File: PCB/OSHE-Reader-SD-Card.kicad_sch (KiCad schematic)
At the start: 2 parts, among them J2 112L-TDA0

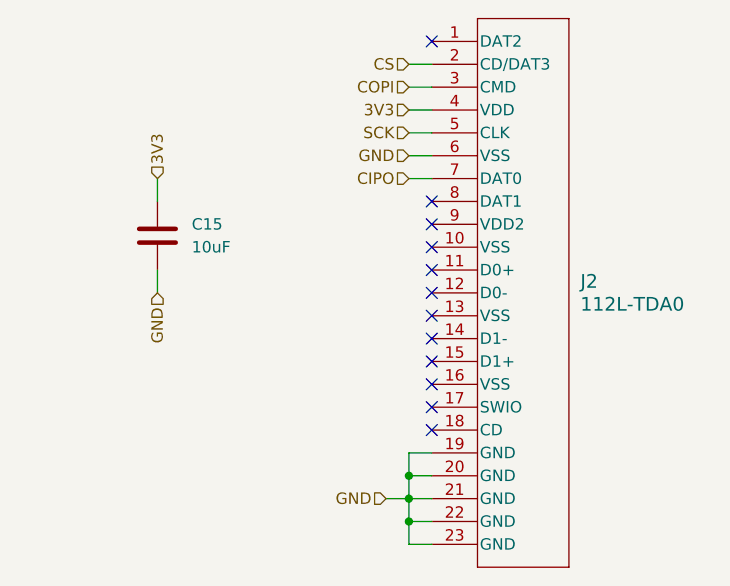
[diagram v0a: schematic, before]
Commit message: HOPEFULLY GOOD FOR EVER (good for first semester) :)
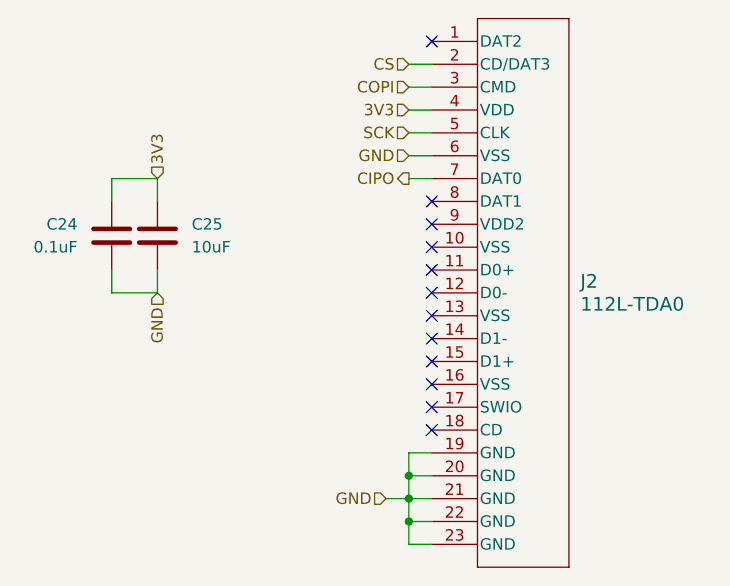
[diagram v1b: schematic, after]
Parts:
- added C24: 0.1uF, symbol Device:C
- J2: footprint CONN_112L-TDA0_ATT -> 112L_TDA0:CONN_112L-TDA0_ATT
- renumbered C15 to C25
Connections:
- net 3V3: now also C24.1
- net GND: now also C24.2
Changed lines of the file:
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@@
+	(wire
+		(pts
+			(xy 39.37 67.31) (xy 39.37 64.77)
+		)
+		(stroke
+			(width 0)
+			(type default)
+		)
+	)
 	(wire
 		(pts
@@
 	(wire
 		(pts
+			(xy 39.37 77.47) (xy 44.45 77.47)
+		)
+		(stroke
+			(width 0)
+			(type default)
+		)
+	)
+	(wire
+		(pts
 			(xy 69.85 100.33) (xy 72.39 100.33)
 		)
@@
 	(wire
 		(pts
+			(xy 39.37 64.77) (xy 44.45 64.77)
+		)
+		(stroke
+			(width 0)
+			(type default)
+		)
+	)
+	(wire
+		(pts
 			(xy 72.39 52.07) (xy 74.93 52.07)
 		)
@@
 	(wire
 		(pts
+			(xy 39.37 74.93) (xy 39.37 77.47)
+		)
+		(stroke
+			(width 0)
+			(type default)
+		)
+	)
+	(wire
+		(pts
 			(xy 72.39 59.69) (xy 74.93 59.69)
 		)
@@
 	)
 	(hierarchical_label "CIPO"
-		(shape input)
+		(shape output)
 		(at 72.39 64.77 180)
 		(effects
@@
 			)
 			(justify right)
+		)
+	)
+	(symbol
+		(lib_id "Device:C")
+		(at 39.37 71.12 0)
+		(mirror y)
+		(unit 1)
+		(exclude_from_sim no)
+		(in_bom yes)
+		(on_board yes)
+		(dnp no)
+		(property "Reference" "C24"
+			(at 35.56 69.8499 0)
+			(effects
+				(font
+					(size 1.27 1.27)
+				)
+				(justify left)
+			)
+		)
+		(property "Value" "0.1uF"
+			(at 35.56 72.3899 0)
+			(effects
+				(font
+					(size 1.27 1.27)
+				)
+				(justify left)
+			)
+		)
+		(property "Footprint" ""
+			(at 38.4048 74.93 0)
+			(effects
+				(font
+					(size 1.27 1.27)
+				)
+				(hide yes)
+			)
+		)
+		(property "Datasheet" "~"
+			(at 39.37 71.12 0)
+			(effects
+				(font
+					(size 1.27 1.27)
+				)
+				(hide yes)
+			)
+		)
+		(property "Description" "Unpolarized capacitor"
+			(at 39.37 71.12 0)
+			(effects
+				(font
+					(size 1.27 1.27)
+				)
+				(hide yes)
+			)
+		)
+		(pin "1"
+		)
+		(pin "2"
+		)
+		(instances
+			(project "OSHE-Reader-PCB"
+				(path "/3f072c92-e35a-4654-839b-728bd3dc3a46/f673c940-d558-4160-83eb-d33ca6356616"
+					(reference "C24")
+					(unit 1)
+				)
+			)
 		)
 	)
@@
 			)
 		)
-		(property "Footprint" "CONN_112L-TDA0_ATT"
+		(property "Footprint" "112L_TDA0:CONN_112L-TDA0_ATT"
 			(at 69.85 49.53 0)
 			(effects
@@
 		(dnp no)
 		(fields_autoplaced yes)
-		(property "Reference" "C15"
+		(property "Reference" "C25"
 			(at 48.26 69.8499 0)
 			(effects
@@
 			(project ""
 				(path "/3f072c92-e35a-4654-839b-728bd3dc3a46/f673c940-d558-4160-83eb-d33ca6356616"
-					(reference "C15")
+					(reference "C25")
 					(unit 1)
 				)

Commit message: small
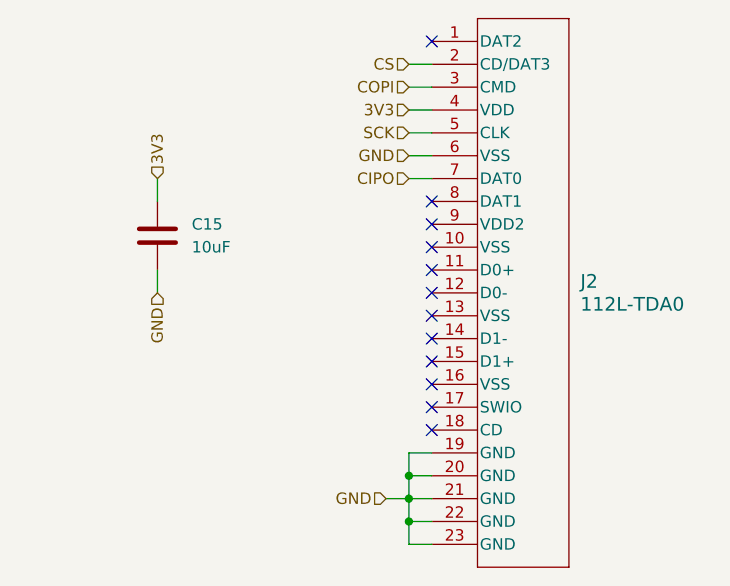
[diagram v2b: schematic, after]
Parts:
- removed C24: 0.1uF, symbol Device:C
- J2: footprint 112L_TDA0:CONN_112L-TDA0_ATT -> CONN_112L-TDA0_ATT
- renumbered C25 to C15
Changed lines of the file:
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@@
-	(wire
-		(pts
-			(xy 39.37 67.31) (xy 39.37 64.77)
-		)
-		(stroke
-			(width 0)
-			(type default)
-		)
-	)
 	(wire
 		(pts
@@
 	(wire
 		(pts
-			(xy 39.37 77.47) (xy 44.45 77.47)
-		)
-		(stroke
-			(width 0)
-			(type default)
-		)
-	)
-	(wire
-		(pts
 			(xy 69.85 100.33) (xy 72.39 100.33)
 		)
@@
 	(wire
 		(pts
-			(xy 39.37 64.77) (xy 44.45 64.77)
-		)
-		(stroke
-			(width 0)
-			(type default)
-		)
-	)
-	(wire
-		(pts
 			(xy 72.39 52.07) (xy 74.93 52.07)
 		)
@@
 	(wire
 		(pts
-			(xy 39.37 74.93) (xy 39.37 77.47)
-		)
-		(stroke
-			(width 0)
-			(type default)
-		)
-	)
-	(wire
-		(pts
 			(xy 72.39 59.69) (xy 74.93 59.69)
 		)
@@
 	)
 	(hierarchical_label "CIPO"
-		(shape output)
+		(shape input)
 		(at 72.39 64.77 180)
 		(effects
@@
 			)
 			(justify right)
-		)
-	)
-	(symbol
-		(lib_id "Device:C")
-		(at 39.37 71.12 0)
-		(mirror y)
-		(unit 1)
-		(exclude_from_sim no)
-		(in_bom yes)
-		(on_board yes)
-		(dnp no)
-		(property "Reference" "C24"
-			(at 35.56 69.8499 0)
-			(effects
-				(font
-					(size 1.27 1.27)
-				)
-				(justify left)
-			)
-		)
-		(property "Value" "0.1uF"
-			(at 35.56 72.3899 0)
-			(effects
-				(font
-					(size 1.27 1.27)
-				)
-				(justify left)
-			)
-		)
-		(property "Footprint" ""
-			(at 38.4048 74.93 0)
-			(effects
-				(font
-					(size 1.27 1.27)
-				)
-				(hide yes)
-			)
-		)
-		(property "Datasheet" "~"
-			(at 39.37 71.12 0)
-			(effects
-				(font
-					(size 1.27 1.27)
-				)
-				(hide yes)
-			)
-		)
-		(property "Description" "Unpolarized capacitor"
-			(at 39.37 71.12 0)
-			(effects
-				(font
-					(size 1.27 1.27)
-				)
-				(hide yes)
-			)
-		)
-		(pin "1"
-		)
-		(pin "2"
-		)
-		(instances
-			(project "OSHE-Reader-PCB"
-				(path "/3f072c92-e35a-4654-839b-728bd3dc3a46/f673c940-d558-4160-83eb-d33ca6356616"
-					(reference "C24")
-					(unit 1)
-				)
-			)
 		)
 	)
@@
 			)
 		)
-		(property "Footprint" "112L_TDA0:CONN_112L-TDA0_ATT"
+		(property "Footprint" "CONN_112L-TDA0_ATT"
 			(at 69.85 49.53 0)
 			(effects
@@
 		(dnp no)
 		(fields_autoplaced yes)
-		(property "Reference" "C25"
+		(property "Reference" "C15"
 			(at 48.26 69.8499 0)
 			(effects
@@
 			(project ""
 				(path "/3f072c92-e35a-4654-839b-728bd3dc3a46/f673c940-d558-4160-83eb-d33ca6356616"
-					(reference "C25")
+					(reference "C15")
 					(unit 1)
 				)
